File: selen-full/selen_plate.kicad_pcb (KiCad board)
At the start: 2 copper layers, 121.3 x 94.1 mm, 8 parts

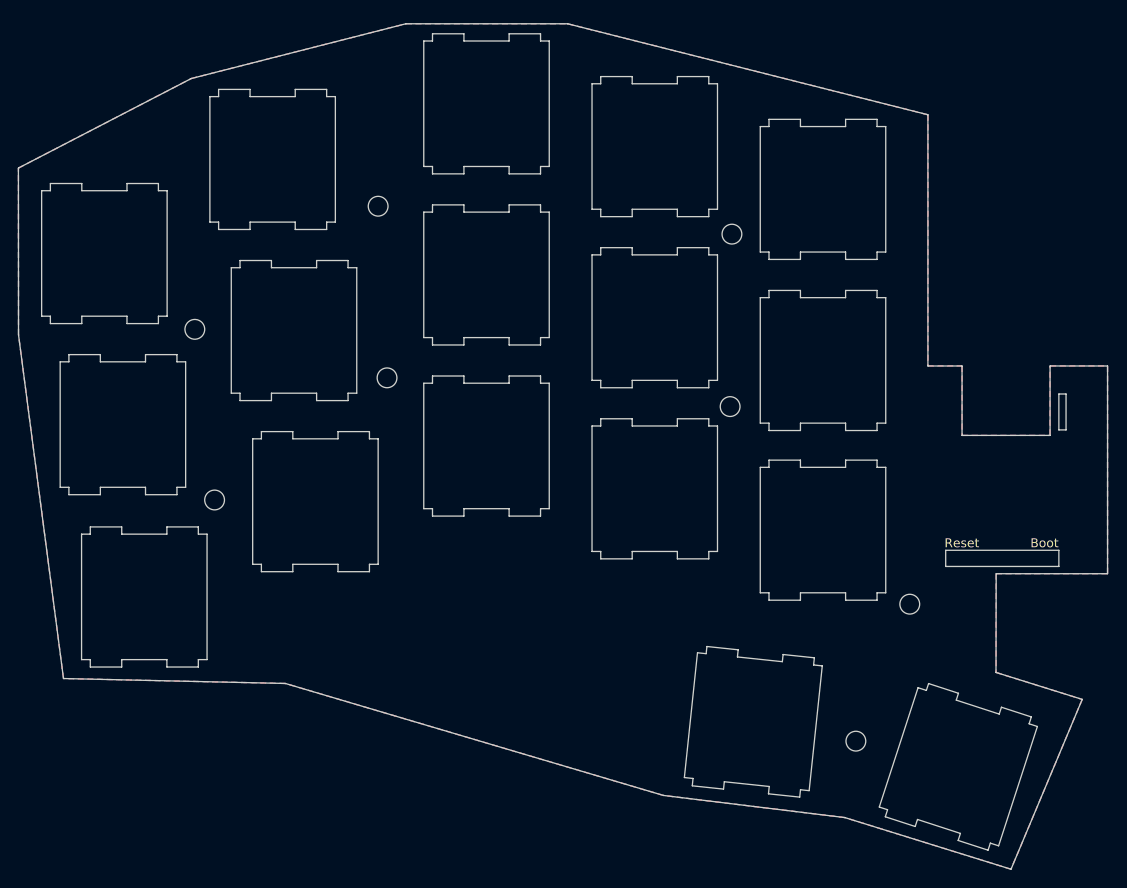
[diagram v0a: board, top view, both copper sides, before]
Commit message: Update plate PCB
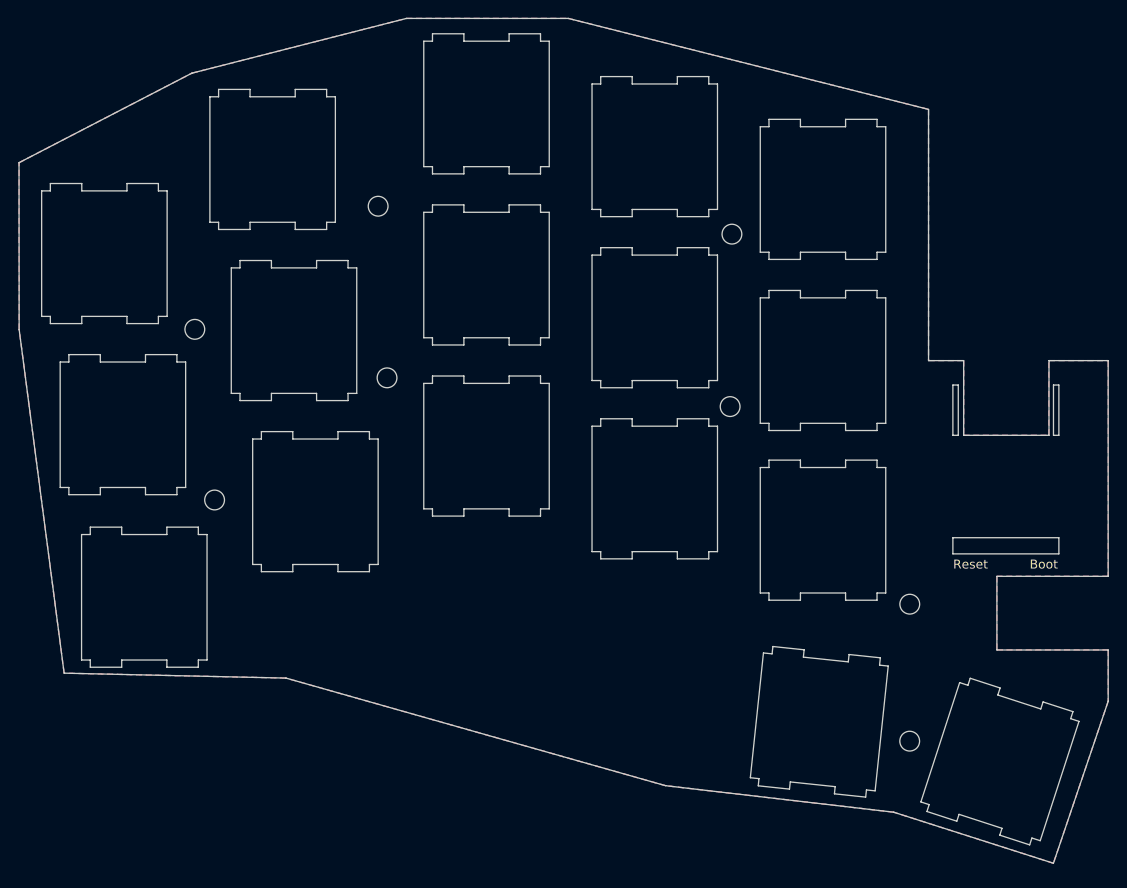
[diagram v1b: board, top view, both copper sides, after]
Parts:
- moved REF** 5.99 mm to (190.0, 135.2)
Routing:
- added copper zone on B.Cu, net (none)
- added copper zone on F.Cu, net (none)
- removed copper zone on B.Cu, net GND
- removed copper zone on F.Cu, net GND
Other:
- outline, holes or cut-outs redrawn
- board text added: "Selen v.0.2.1"
- board text removed: "Selen v.0.2.0"
